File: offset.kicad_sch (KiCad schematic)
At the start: 35 parts, among them U11 OPA2189D, U18 TMUX6219DGK, U19 TCA0372

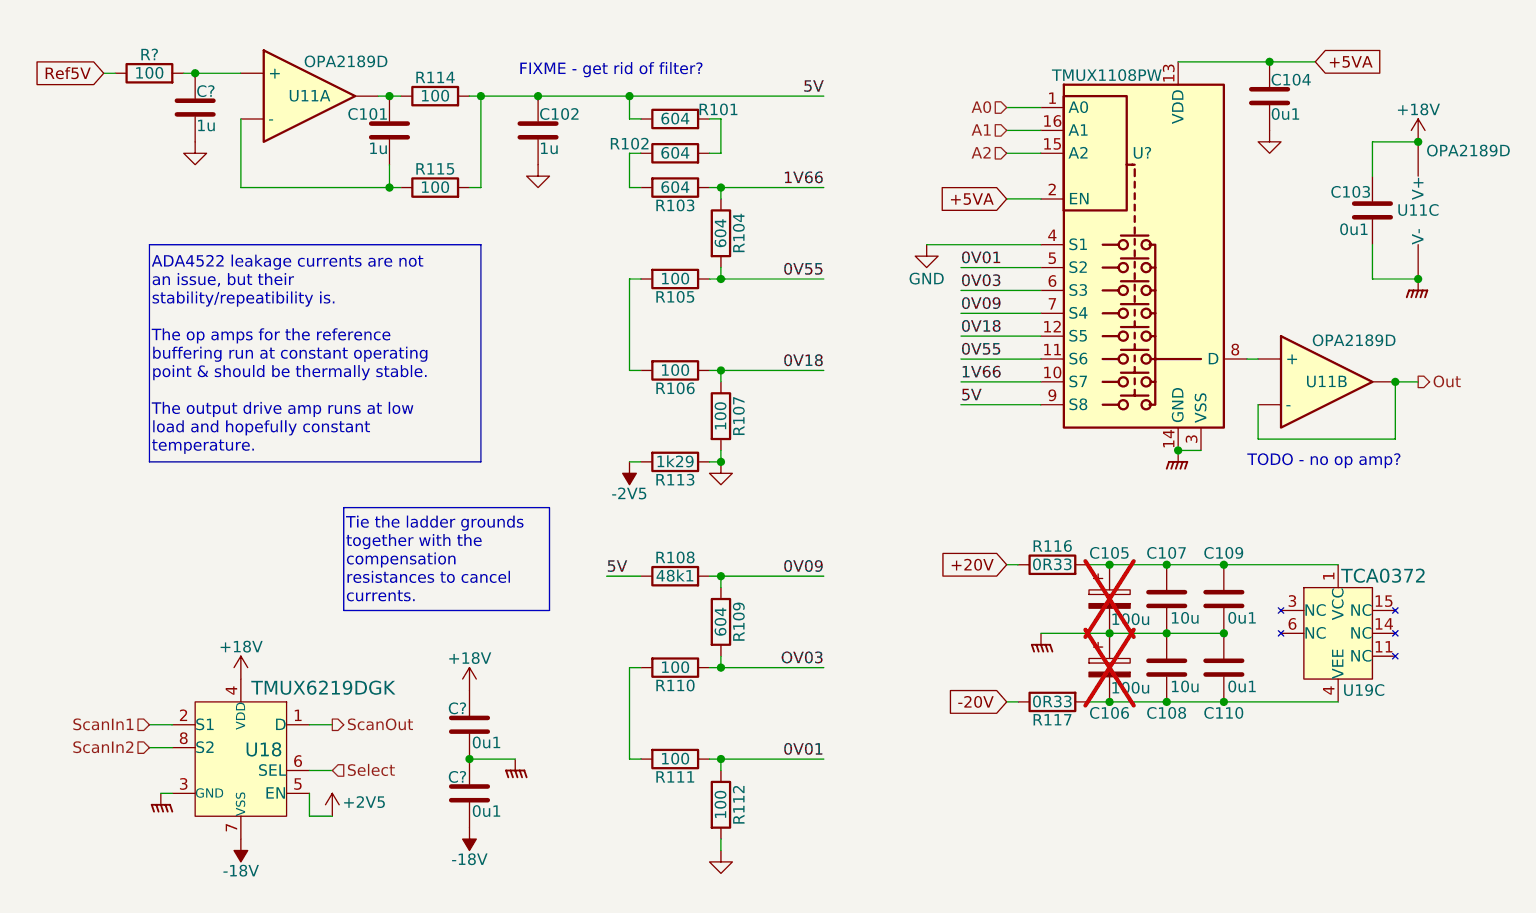
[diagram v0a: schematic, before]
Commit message: Schematic complete, maybe
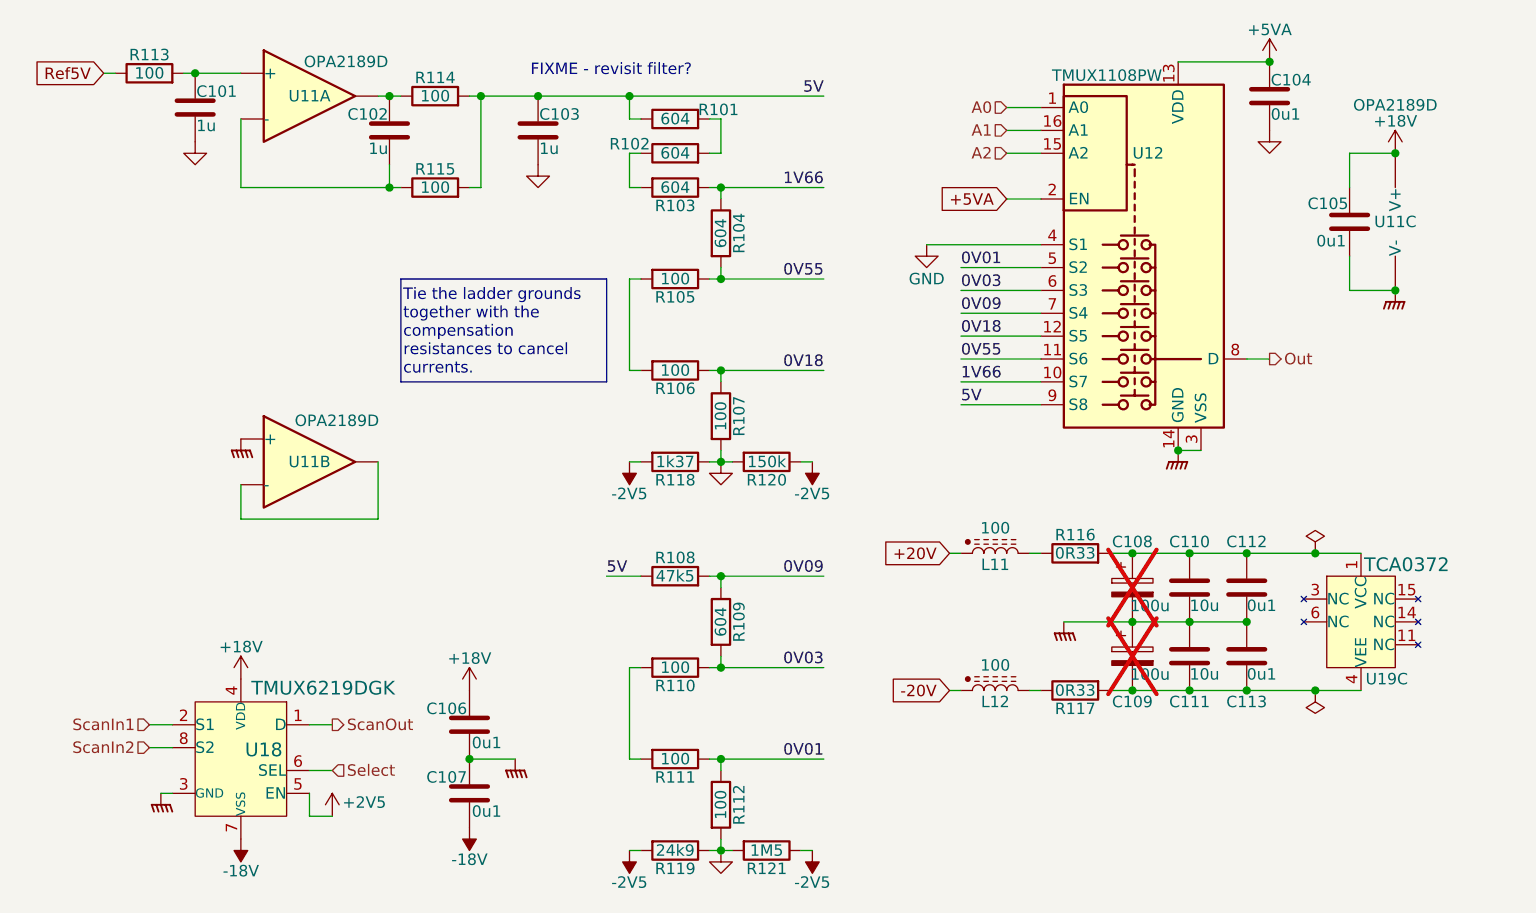
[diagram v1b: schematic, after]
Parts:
- added L11, L12: 100, Inductor_SMD:L_0603_1608Metric, symbol Parts:L_Ferrite_Power
- added R119: 24k9, Resistor_SMD:R_0603_1608Metric, symbol Device:R
- added R120: 150k, Resistor_SMD:R_0603_1608Metric, symbol Device:R
- added R121: 1M5, Resistor_SMD:R_0603_1608Metric, symbol Device:R
- C101: renamed from C?; footprint (none) -> Capacitor_SMD:C_0402_1005Metric; LCSC (none) -> C52923
- C102: renamed from C101; footprint (none) -> Capacitor_SMD:C_0402_1005Metric; LCSC (none) -> C52923
- C103: renamed from C102; footprint (none) -> Capacitor_SMD:C_0402_1005Metric; LCSC (none) -> C52923
- C104: footprint (none) -> Capacitor_SMD:C_0402_1005Metric; LCSC (none) -> C307331
- C105: renamed from C103; footprint (none) -> Capacitor_SMD:C_0402_1005Metric; LCSC (none) -> C307331
- C106, C107: renamed from C?; footprint (none) -> Capacitor_SMD:C_0402_1005Metric; LCSC (none) -> C307331
- C108: renamed from C105; now left out of the parts list
- C109: renamed from C106; now left out of the parts list
- C110: renamed from C107; footprint (none) -> Capacitor_SMD:C_0805_2012Metric; LCSC (none) -> C440198
- C111: renamed from C108; footprint (none) -> Capacitor_SMD:C_0805_2012Metric; LCSC (none) -> C440198
- C112: renamed from C109; footprint (none) -> Capacitor_SMD:C_0402_1005Metric; LCSC (none) -> C307331
- C113: renamed from C110; footprint (none) -> Capacitor_SMD:C_0402_1005Metric; LCSC (none) -> C307331
- R101, R102, R103, R104, R105, R106, R107, R109, R110, R111, R112, U19: now left out of the parts list
- R108: value 48k1 -> 47k5; now left out of the parts list
- R118: renamed from R113; value 1k29 -> 1k37
- U11: LCSC (none) -> C881489; now left out of the parts list
- U12: renamed from U?; LCSC (none) -> C1021800; now left out of the parts list
- U18: LCSC (none) -> C2876423
- gave numbers to parts that had none: 1
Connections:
- net OV03 is gone; now on net 0V03: R109.2, R110.1
- net +20V: now also L11.1; no longer R116.1
- net -20V: now also L12.1; no longer R117.1
- net -2V5: now also R119.2, R120.1, R121.1
- net GND: now also R119.1, R120.2, R121.2
- net GNDPWR: now also U11.5 (+)
- net Out: now also U12.8 (D); no longer U11.6 (-), U11.7
- new net: L12.2, R117.1
- new net: L11.2, R116.1
- new net: U11.6 (-), U11.7
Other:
- note added: "FIXME - revisit filter?"
- note removed: "FIXME - get rid of filter?"
- note removed: "TODO - no op amp?"
- moved on the sheet: C105, C108, C109, C110, C111, C112, C113, R116, R117, U11B, U11C, U19C

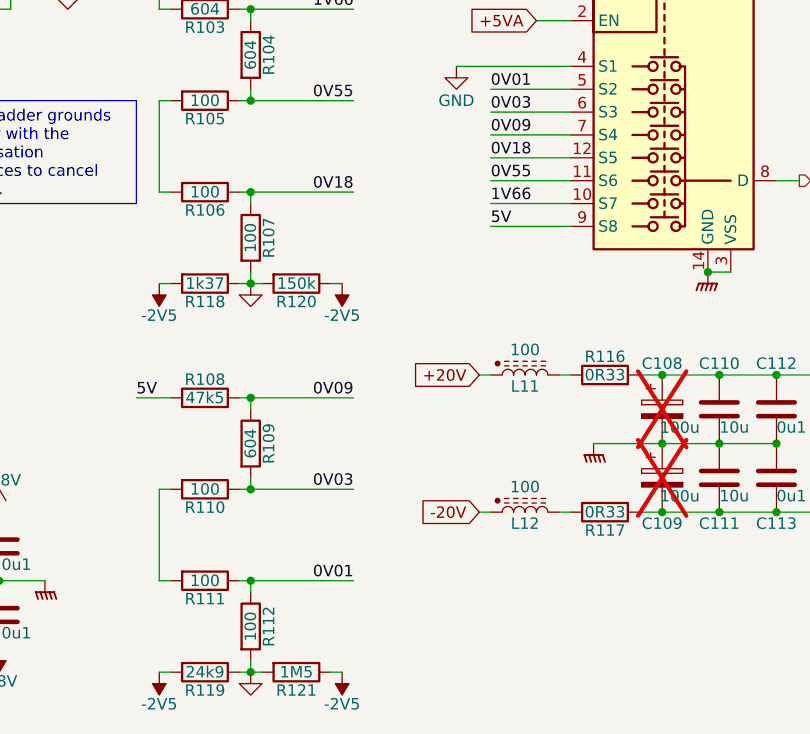
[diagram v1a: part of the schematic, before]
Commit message: Part selection
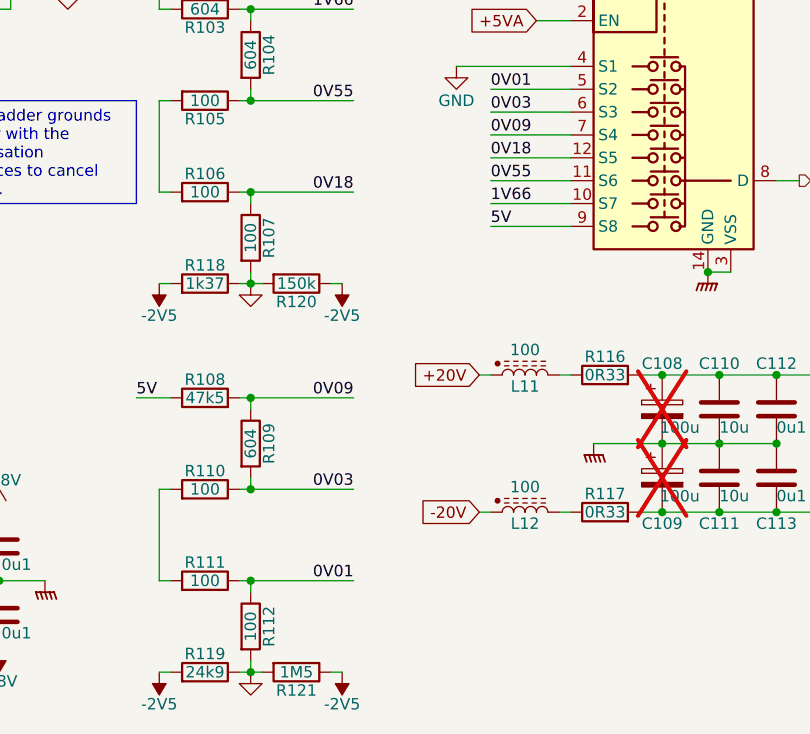
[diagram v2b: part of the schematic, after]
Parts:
- R113, R114, R115: LCSC (none) -> C25076
- R116, R117, R118, R119: now left out of the parts list
- R120: LCSC (none) -> C22807
- R121: LCSC (none) -> C4172
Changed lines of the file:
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@@
 		(lib_id "Device:R")
 		(at 128.27 143.51 270)
+		(mirror x)
 		(unit 1)
 		(exclude_from_sim no)
-		(in_bom yes)
+		(in_bom no)
 		(on_board yes)
 		(dnp no)
 		(property "Reference" "R119"
-			(at 128.27 145.542 90)
+			(at 128.27 141.478 90)
 			(effects
 				(font
@@
 		)
 		(property "Footprint" "Resistor_SMD:R_0603_1608Metric"
-			(at 128.27 141.732 90)
+			(at 128.27 145.288 90)
 			(effects
 				(font
@@
 		(lib_id "Device:R")
 		(at 172.72 125.73 90)
-		(mirror x)
 		(unit 1)
 		(exclude_from_sim no)
-		(in_bom yes)
+		(in_bom no)
 		(on_board yes)
 		(dnp no)
 		(property "Reference" "R117"
-			(at 172.72 127.762 90)
+			(at 172.72 123.698 90)
 			(effects
 				(font
@@
 		)
 		(property "Footprint" "Resistor_SMD:R_0805_2012Metric"
-			(at 172.72 123.952 90)
+			(at 172.72 127.508 90)
 			(effects
 				(font
@@
 		(lib_id "Device:R")
 		(at 128.27 90.17 270)
+		(mirror x)
 		(unit 1)
 		(exclude_from_sim no)
@@
 		(dnp no)
 		(property "Reference" "R106"
-			(at 128.27 92.202 90)
+			(at 128.27 88.138 90)
 			(effects
 				(font
@@
 		)
 		(property "Footprint" "Resistor_SMD:R_0603_1608Metric"
-			(at 128.27 88.392 90)
+			(at 128.27 91.948 90)
 			(effects
 				(font
@@
 			)
 		)
+		(property "LCSC" "C25076"
+			(at 101.6 59.69 90)
+			(effects
+				(font
+					(size 1.27 1.27)
+				)
+				(hide yes)
+			)
+		)
 		(pin "1"
 		)
@@
 		(lib_id "Device:R")
 		(at 128.27 100.33 270)
+		(mirror x)
 		(unit 1)
 		(exclude_from_sim no)
-		(in_bom yes)
+		(in_bom no)
 		(on_board yes)
 		(dnp no)
 		(property "Reference" "R118"
-			(at 128.27 102.362 90)
+			(at 128.27 98.298 90)
 			(effects
 				(font
@@
 		)
 		(property "Footprint" "Resistor_SMD:R_0603_1608Metric"
-			(at 128.27 98.552 90)
+			(at 128.27 102.108 90)
 			(effects
 				(font
@@
 		(lib_id "Device:R")
 		(at 128.27 133.35 270)
+		(mirror x)
 		(unit 1)
 		(exclude_from_sim no)
@@
 		(dnp no)
 		(property "Reference" "R111"
-			(at 128.27 135.382 90)
+			(at 128.27 131.318 90)
 			(effects
 				(font
@@
 		)
 		(property "Footprint" "Resistor_SMD:R_0603_1608Metric"
-			(at 128.27 131.572 90)
+			(at 128.27 135.128 90)
 			(effects
 				(font
@@
 		(unit 1)
 		(exclude_from_sim no)
-		(in_bom yes)
+		(in_bom no)
 		(on_board yes)
 		(dnp no)
@@
 		(lib_id "Device:R")
 		(at 128.27 123.19 270)
+		(mirror x)
 		(unit 1)
 		(exclude_from_sim no)
@@
 		(dnp no)
 		(property "Reference" "R110"
-			(at 128.27 125.222 90)
+			(at 128.27 121.158 90)
 			(effects
 				(font
@@
 		)
 		(property "Footprint" "Resistor_SMD:R_0603_1608Metric"
-			(at 128.27 121.412 90)
+			(at 128.27 124.968 90)
 			(effects
 				(font
@@
 			)
 		)
+		(property "LCSC" "C22807"
+			(at 138.43 100.33 90)
+			(effects
+				(font
+					(size 1.27 1.27)
+				)
+				(hide yes)
+			)
+		)
 		(pin "2"
 		)
@@
 			)
 		)
+		(property "LCSC" "C4172"
+			(at 138.43 143.51 90)
+			(effects
+				(font
+					(size 1.27 1.27)
+				)
+				(hide yes)
+			)
+		)
 		(pin "2"
 		)
@@
 			)
 		)
+		(property "LCSC" "C25076"
+			(at 69.85 57.15 90)
+			(effects
+				(font
+					(size 1.27 1.27)
+				)
+				(hide yes)
+			)
+		)
 		(pin "1"
 		)
@@
 			(effects
 				(font
+					(size 1.27 1.27)
+				)
+				(hide yes)
+			)
+		)
+		(property "LCSC" "C25076"
+			(at 101.6 69.85 90)
+			(effects
+				(font

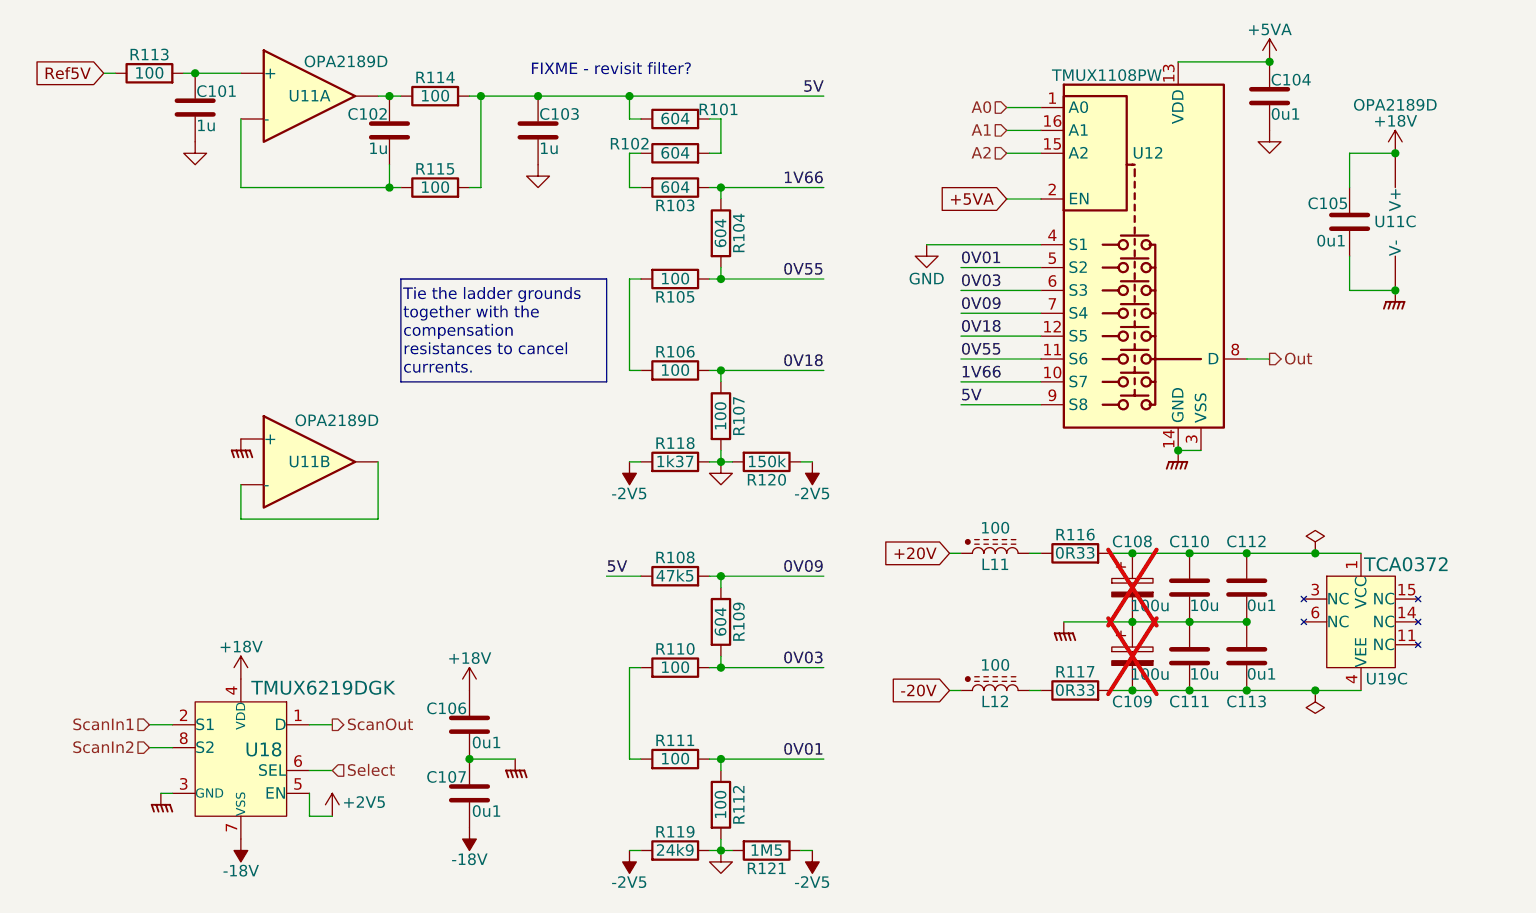
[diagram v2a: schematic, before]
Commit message: ERC passes.
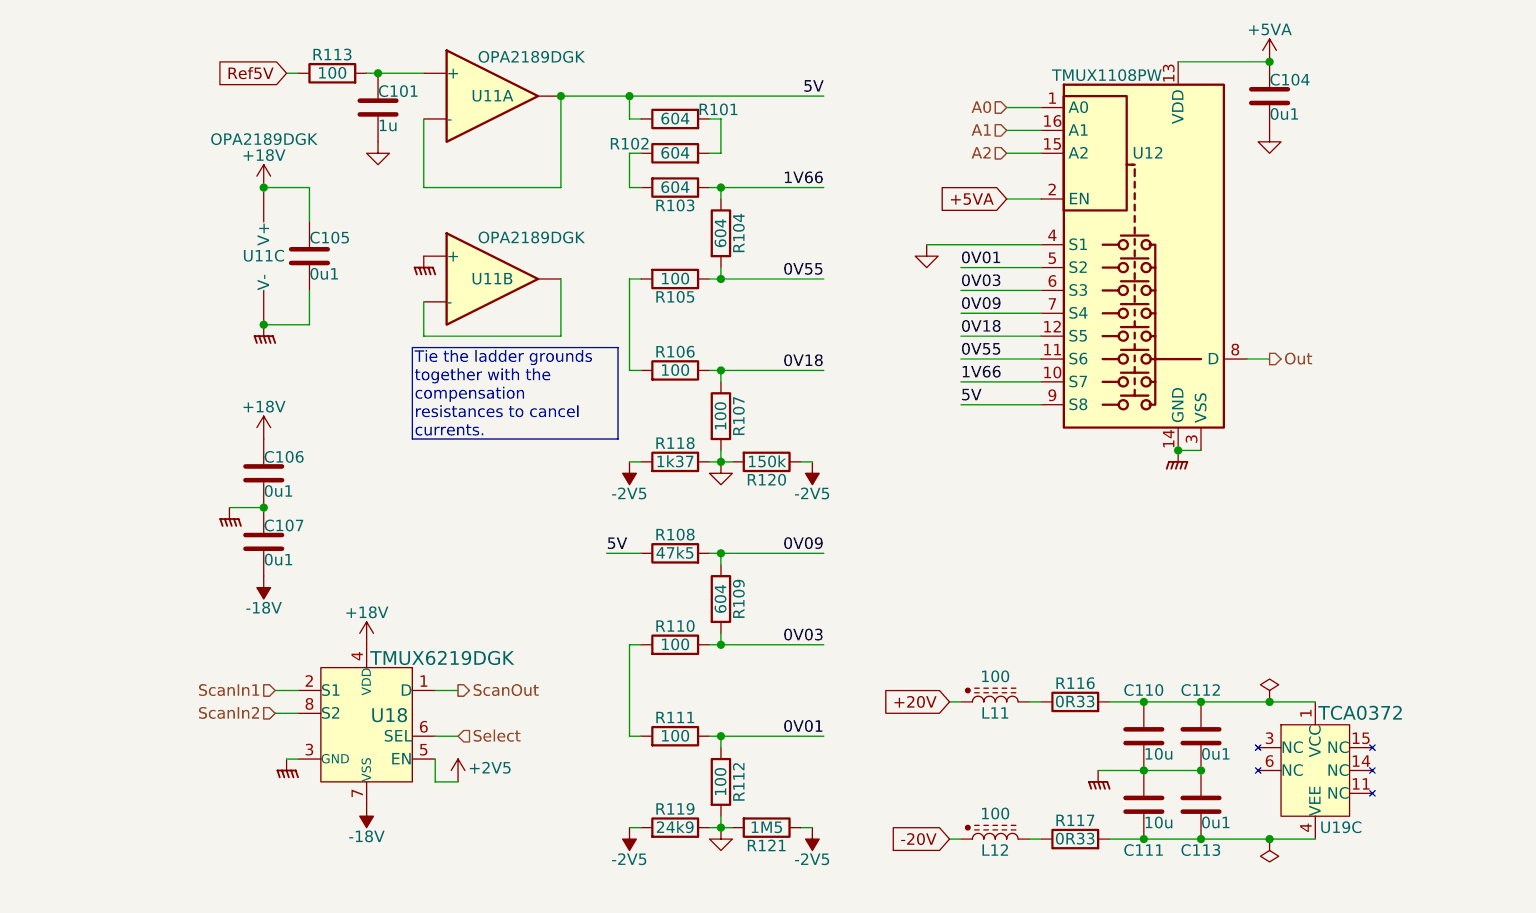
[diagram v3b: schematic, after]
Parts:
- removed C102, C103: 1u, Capacitor_SMD:C_0402_1005Metric, symbol Device:C
- removed C108, C109: 100u, symbol Device:C_Polarized
- removed R114, R115: 100, Resistor_SMD:R_0402_1005Metric, symbol Device:R
- U11: value OPA2189D -> OPA2189DGK; footprint Package_SO:SOIC-8_3.9x4.9mm_P1.27mm -> Package_SO:MSOP-8_3x3mm_P0.65mm; symbol Parts:OPA2189D -> Parts:OPA2189DGK
- U18: footprint SOIC8_DGK_TEX -> Package_SO:VSSOP-8_3x3mm_P0.65mm
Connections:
- net 5V: now also U11.1, U11.2 (-)
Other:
- note removed: "FIXME - revisit filter?"
- moved on the sheet: C101, C105, C106, C107, C110, C111, C112, C113, L11, L12, R108, R109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
